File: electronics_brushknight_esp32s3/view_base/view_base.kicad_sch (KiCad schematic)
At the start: 107 parts, among them J1 BLDC, J2 USB_C_Receptacle_USB2.0, J3 LCD, J4 A, J5 B, Q1 MMBT4403, Q2 UMH3N, U1 MT6701-CT, U10 ESP32-S3-WROOM-1-N8R8, U4 CP2102N-A02-GQFN28, U4 HX711, U5 TMC6300, U7 SN74LV1T34DBV, U8 VEML7700, U9 TS1117BCW33_RPG

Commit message: devkit pcb preview
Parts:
- removed D1, D2, D3, D4, D5, D6, D7, D8: SK6812SIDE-A, cleaned footprints:SK6812-SIDE-A, symbol SK6812:SK6812SIDE-A
- removed H4: MountHole, Holes:MountingHole_2.2mm_M2_ISO7380_Pad_NonVirtual, symbol Mechanical:MountingHole_Pad
- removed Q2: UMH3N, cleaned footprints:SOT-363_SC-70-6, symbol Transistor_BJT:UMH3N
- removed R3: 1K, cleaned footprints:R_0603_1608Metric, symbol Device:R_Small
- removed U4: CP2102N-A02-GQFN28, cp2102:Silicon_Labs-CP2102N-A02-GQFN28-IPC_A, symbol terrarium-rescue:CP2102N-A02-GQFN28-CP2102N-A02-GQFN28
- added C100, C101, C30, C31, C32, C33, C34, C35, C36, C37, C38, C39, C40, C41, C42, C43, C44, C45, C46, C47, C48, C49, C50, C51, C52, C53, C54, C55, C56, C57, C58, C59, C60, C61, C62, C63, C64, C65, C66, C67, C68, C69, C70, C71, C72, C73, C74, C75, C76, C77, C79, C80, C81, C82, C88, C90, C92, C94, C95, C96, C97, C98, C99: 0.1uF, cleaned footprints:C_0402_1005Metric, symbol Device:C_Small
- added C27, C38: 10uF, smd_clean:C_0603_1608Metric, symbol Device:C_Small
- added C39: 100nF, smd_clean:C_0603_1608Metric, symbol Device:C_Small
- added D10, D11, D12, D13, D14, D15, D16, D17, D18, D19, D20, D21, D22, D23, D24, D25, D26, D27, D28, D29, D30, D31, D32, D33, D34, D35, D36, D37, D38, D39, D40, D41, D42, D43, D44, D45, D46, D47, D48, D49, D50, D51, D52, D53, D54, D55, D56, D57, D58, D59, D60, D61, D62, D63, D64, D65, D66, D67, D68, D69, D70, D71, D72, D73, D74, D75, D76, D77, D78, D79, D80, D9: SK6805, cleaned footprints:LED_SK6812_EC15_1.5x1.5mm, symbol LED:SK6812
- added J6: LCD - FPC, screen_connector:Amphenol FCI FPC 8 pin 0.5 pitch, symbol Connector_Generic:Conn_01x08
- added J7, J8, J9: Conn_01x04_Socket, cleaned footprints:JST_SH_SM04B-SRSS-TB_1x04-1MP_P1.00mm_Horizontal, symbol Connector:Conn_01x04_Socket
- added Q4, Q5: BSS138, smd_clean:SOT-23, symbol Transistor_FET:BSS138
- added R18, R19, R20, R21, R22, R23: 10K, smd_clean:R_0603_1608Metric, symbol Device:R_Small
- added R28: 10k, cleaned footprints:R_0603_1608Metric, symbol Device:R_Small
- added SW1: RST, smd_clean:SW_SPST_PTS810, symbol Switch:SW_Push
- added SW2: Boot, smd_clean:SW_SPST_PTS810, symbol Switch:SW_Push
- added TP17: IO40, cleaned footprints:TestPoint_Pad_D2.0mm_ValueSilk, symbol Connector:TestPoint_Small
- added TP18: IO41, cleaned footprints:TestPoint_Pad_D2.0mm_ValueSilk, symbol Connector:TestPoint_Small
- added TP19: IO42, cleaned footprints:TestPoint_Pad_D2.0mm_ValueSilk, symbol Connector:TestPoint_Small
- added TP20: IO45, cleaned footprints:TestPoint_Pad_D2.0mm_ValueSilk, symbol Connector:TestPoint_Small
- added TP21: IO46, cleaned footprints:TestPoint_Pad_D2.0mm_ValueSilk, symbol Connector:TestPoint_Small
- added TP22: IO47, cleaned footprints:TestPoint_Pad_D2.0mm_ValueSilk, symbol Connector:TestPoint_Small
- added TP23: IO48, cleaned footprints:TestPoint_Pad_D2.0mm_ValueSilk, symbol Connector:TestPoint_Small
- added U2: USBLC6-2SC6, smd_clean:SOT-23-6, symbol Power_Protection:USBLC6-2SC6
- added U7: VL53L0CXV0DH_1, smd_clean:LGA12_1, symbol VL53L0CXV0DH_1:VL53L0CXV0DH_1
- added U8: LP5907MFX-2.8, cleaned footprints:SOT-23-5, symbol Regulator_Linear:LP5907MFX-2.8
- C1, C11, C2, C29, C3, C4, C5, C6, C7, C8: footprint cleaned footprints:C_0603_1608Metric -> cleaned footprints:C_0402_1005Metric; Digikey 1276-1935-1-ND -> (none); LCSC C1591 -> C83056; Mouser 187-CL10B104KB8NNWC -> (none)
- TP1, TP10, TP11, TP12, TP13, TP14, TP15, TP16, TP3, TP4, TP5, TP6, TP7, TP8, TP9: footprint Modified:TestPoint_Pad_D2.0mm_ValueSilk -> cleaned footprints:TestPoint_Pad_D2.0mm_ValueSilk
- TP2: value 3.3v -> 3V3; footprint Modified:TestPoint_Pad_D2.0mm_ValueSilk -> cleaned footprints:TestPoint_Pad_D2.0mm_ValueSilk
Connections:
- net +3V3: now also C27.2, J6.1 (Pin_1), R20.2, R21.2, R28.1, U8.1 (IN), U8.3 (EN); no longer C11.1
- net +5V: now also C11.1, C100.1, C101.1, C30.1, C31.1, C32.1, C33.1, C34.1, C35.1, C36.1, C37.1, C38.1, C39.1, C40.1, C41.1, C42.1, C43.1, C44.1, C45.1, C46.1, C47.1, C48.1, C49.1, C50.1, C51.1, C52.1, C53.1, C54.1, C55.1, C56.1, C57.1, C58.1, C59.1, C60.1, C61.1, C62.1, C63.1, C64.1, C65.1, C66.1, C67.1, C68.1, C69.1, C70.1, C71.1, C72.1, C73.1, C74.1, C75.1, C76.1, C77.1, C79.1, C80.1, C81.1, C82.1, C88.1, C90.1, C92.1, C94.1, C95.1, C96.1, C97.1, C98.1, C99.1, D10.3 (VDD), D11.3 (VDD), D12.3 (VDD), D13.3 (VDD), D14.3 (VDD), D15.3 (VDD), D16.3 (VDD), D17.3 (VDD), D18.3 (VDD), D19.3 (VDD), D20.3 (VDD), D21.3 (VDD), D22.3 (VDD), D23.3 (VDD), D24.3 (VDD), D25.3 (VDD), D26.3 (VDD), D27.3 (VDD), D28.3 (VDD), D29.3 (VDD), D30.3 (VDD), D31.3 (VDD), D32.3 (VDD), D33.3 (VDD), D34.3 (VDD), D35.3 (VDD), D36.3 (VDD), D37.3 (VDD), D38.3 (VDD), D39.3 (VDD), D40.3 (VDD), D41.3 (VDD), D42.3 (VDD), D43.3 (VDD), D44.3 (VDD), D45.3 (VDD), D46.3 (VDD), D47.3 (VDD), D48.3 (VDD), D49.3 (VDD), D50.3 (VDD), D51.3 (VDD), D52.3 (VDD), D53.3 (VDD), D54.3 (VDD), D55.3 (VDD), D56.3 (VDD), D57.3 (VDD), D58.3 (VDD), D59.3 (VDD), D60.3 (VDD), D61.3 (VDD), D62.3 (VDD), D63.3 (VDD), D64.3 (VDD), D65.3 (VDD), D66.3 (VDD), D67.3 (VDD), D68.3 (VDD), D69.3 (VDD), D70.3 (VDD), D71.3 (VDD), D72.3 (VDD), D73.3 (VDD), D74.3 (VDD), D75.3 (VDD), D76.3 (VDD), D77.3 (VDD), D78.3 (VDD), D79.3 (VDD), D80.3 (VDD), D9.3 (VDD), J7.3 (Pin_3), J8.3 (Pin_3), J9.3 (Pin_3), U2.5 (VBUS)
- net ESP32_BOOT: now also R28.2, SW2.1
- net ESP32_EN: now also SW1.1
- net GND: now also C100.2, C101.2, C27.1, C30.2, C31.2, C32.2, C33.2, C34.2, C35.2, C36.2, C37.2, C38.1, C38.2, C39.1, C39.2, C40.2, C41.2, C42.2, C43.2, C44.2, C45.2, C46.2, C47.2, C48.2, C49.2, C50.2, C51.2, C52.2, C53.2, C54.2, C55.2, C56.2, C57.2, C58.2, C59.2, C60.2, C61.2, C62.2, C63.2, C64.2, C65.2, C66.2, C67.2, C68.2, C69.2, C70.2, C71.2, C72.2, C73.2, C74.2, C75.2, C76.2, C77.2, C79.2, C80.2, C81.2, C82.2, C88.2, C90.2, C92.2, C94.2, C95.2, C96.2, C97.2, C98.2, C99.2, D10.1 (VSS), D11.1 (VSS), D12.1 (VSS), D13.1 (VSS), D14.1 (VSS), D15.1 (VSS), D16.1 (VSS), D17.1 (VSS), D18.1 (VSS), D19.1 (VSS), D20.1 (VSS), D21.1 (VSS), D22.1 (VSS), D23.1 (VSS), D24.1 (VSS), D25.1 (VSS), D26.1 (VSS), D27.1 (VSS), D28.1 (VSS), D29.1 (VSS), D30.1 (VSS), D31.1 (VSS), D32.1 (VSS), D33.1 (VSS), D34.1 (VSS), D35.1 (VSS), D36.1 (VSS), D37.1 (VSS), D38.1 (VSS), D39.1 (VSS), D40.1 (VSS), D41.1 (VSS), D42.1 (VSS), D43.1 (VSS), D44.1 (VSS), D45.1 (VSS), D46.1 (VSS), D47.1 (VSS), D48.1 (VSS), D49.1 (VSS), D50.1 (VSS), D51.1 (VSS), D52.1 (VSS), D53.1 (VSS), D54.1 (VSS), D55.1 (VSS), D56.1 (VSS), D57.1 (VSS), D58.1 (VSS), D59.1 (VSS), D60.1 (VSS), D61.1 (VSS), D62.1 (VSS), D63.1 (VSS), D64.1 (VSS), D65.1 (VSS), D66.1 (VSS), D67.1 (VSS), D68.1 (VSS), D69.1 (VSS), D70.1 (VSS), D71.1 (VSS), D72.1 (VSS), D73.1 (VSS), D74.1 (VSS), D75.1 (VSS), D76.1 (VSS), D77.1 (VSS), D78.1 (VSS), D79.1 (VSS), D80.1 (VSS), D9.1 (VSS), J6.2 (Pin_2), J7.4 (Pin_4), J8.4 (Pin_4), J9.4 (Pin_4), SW1.2, SW2.2, U2.2 (GND), U7.12 (GND4), U7.2 (AVSSVCSEL), U7.3 (GND), U7.4 (GND2), U7.6 (GND3), U8.2 (GND)
- net LCD_BACKLIGHT: now also J6.6 (Pin_6)
- net LCD_CMD: now also J6.8 (Pin_8)
- net LCD_CS: now also J6.7 (Pin_7)
- net LCD_DATA: now also J6.5 (Pin_5)
- net LCD_RST: now also U10.18 (IO10), J6.3 (Pin_3); no longer U10.6 (IO6)
- net LCD_SCK: now also J6.4 (Pin_4)
- net LED_DATA_3V3: now also U10.20 (IO12); no longer U10.7 (IO7)
- net LED_DATA_5V: now also D9.2 (DIN)
- net MAG_CSN: now also U10.19 (IO11); no longer U10.22 (IO14)
- net MAG_DO: now also U10.22 (IO14); no longer U10.30 (IO37)
- net SCL: now also U10.31 (IO38), J7.1 (Pin_1), J8.1 (Pin_1), J9.1 (Pin_1), Q4.3 (D), R21.1; no longer U10.12 (IO8)
- net SDA: now also U10.32 (IO39), J7.2 (Pin_2), J8.2 (Pin_2), J9.2 (Pin_2), Q5.3 (D), R20.1; no longer U10.8 (IO15)
- net STRAIN_DO: now also U10.23 (IO21); no longer U10.31 (IO38)
- net TMC_DIAG: now also U10.6 (IO6); no longer U10.29 (IO36)
- net TMC_UH: now also U10.12 (IO8); no longer U10.14 (IO20)
- net TMC_UL: now also U10.9 (IO16); no longer U10.13 (IO19)
- net TMC_VH: now also U10.11 (IO18); no longer U10.23 (IO21)
- net TMC_VL: now also U10.7 (IO7); no longer U10.10 (IO17)
- net TMC_WH: now also U10.10 (IO17); no longer U10.20 (IO12)
- net TMC_WL: now also U10.8 (IO15); no longer U10.11 (IO18)
- net USB_D+: now also U2.3 (I/O2)
- net USB_D-: now also U2.1 (I/O1)
- net at U10.16 (IO46): now also TP21.1
- net at U10.24 (IO47): now also TP22.1
- net at U10.25 (IO48): now also TP23.1
- net at U10.26 (IO45): now also TP20.1
- net at U10.33 (IO40): now also TP17.1
- net at U10.34 (IO41): now also TP18.1
- net at U10.35 (IO42): now also TP19.1
- new net: D27.4 (DOUT), D28.2 (DIN)
- new net: D28.4 (DOUT), D29.2 (DIN)
- new net: D19.4 (DOUT), D20.2 (DIN)
- new net: D20.4 (DOUT), D21.2 (DIN)
- new net: D16.4 (DOUT), D17.2 (DIN)
- new net: D17.4 (DOUT), D18.2 (DIN)
- new net: D34.4 (DOUT), D35.2 (DIN)
- new net: D35.4 (DOUT), D36.2 (DIN)
- new net: D36.4 (DOUT), D37.2 (DIN)
- new net: R19.1, U7.7 (GPIO1)
- new net: D48.4 (DOUT), D52.2 (DIN)
- new net: D52.4 (DOUT), D56.2 (DIN)
- new net: D59.4 (DOUT), D63.2 (DIN)
- new net: D63.4 (DOUT), D67.2 (DIN)
- new net: R18.1, U7.5 (XSHUT)
- new net: D40.4 (DOUT), D41.2 (DIN)
- new net: D41.4 (DOUT), D45.2 (DIN)
- new net: D74.4 (DOUT), D75.2 (DIN)
- new net: D75.4 (DOUT), D76.2 (DIN)
- new net: D24.4 (DOUT), D25.2 (DIN)
- new net: D25.4 (DOUT), D26.2 (DIN)
- new net: D64.4 (DOUT), D68.2 (DIN)
- new net: D68.4 (DOUT), D72.2 (DIN)
- new net: D56.4 (DOUT), D60.2 (DIN)
- new net: D60.4 (DOUT), D64.2 (DIN)
- new net: D49.4 (DOUT), D53.2 (DIN)
- new net: D53.4 (DOUT), D57.2 (DIN)
- new net: D12.4 (DOUT), D13.2 (DIN)
- new net: D13.4 (DOUT), D14.2 (DIN)
- new net: D14.4 (DOUT), D15.2 (DIN)
- new net: D15.4 (DOUT), D16.2 (DIN)
- new net: D61.4 (DOUT), D65.2 (DIN)
- new net: D65.4 (DOUT), D69.2 (DIN)
- new net: D67.4 (DOUT), D71.2 (DIN)
- new net: D44.2 (DIN), D71.4 (DOUT)
- new net: D18.4 (DOUT), D19.2 (DIN)
- new net: D76.4 (DOUT), D77.2 (DIN)
- new net: D77.4 (DOUT), D78.2 (DIN)
- new net: D42.2 (DIN), D69.4 (DOUT)
- new net: D42.4 (DOUT), D46.2 (DIN)
- new net: D46.4 (DOUT), D50.2 (DIN)
- new net: D50.4 (DOUT), D54.2 (DIN)
- new net: D30.4 (DOUT), D31.2 (DIN)
- new net: D31.4 (DOUT), D32.2 (DIN)
- new net: D55.4 (DOUT), D59.2 (DIN)
- new net: D33.4 (DOUT), D34.2 (DIN)
- new net: D26.4 (DOUT), D27.2 (DIN)
- new net: D21.4 (DOUT), D22.2 (DIN)
- new net: D22.4 (DOUT), D23.2 (DIN)
- new net: D44.4 (DOUT), D48.2 (DIN)
- new net: D23.4 (DOUT), D24.2 (DIN)
- new net: D29.4 (DOUT), D30.2 (DIN)
- new net: D78.4 (DOUT), D79.2 (DIN)
- new net: D79.4 (DOUT), D80.2 (DIN)
- new net: D43.4 (DOUT), D47.2 (DIN)
- new net: D47.4 (DOUT), D51.2 (DIN)
- new net: D32.4 (DOUT), D33.2 (DIN)
- new net: D58.4 (DOUT), D62.2 (DIN)
- new net: D62.4 (DOUT), D66.2 (DIN)
- new net: D73.4 (DOUT), D74.2 (DIN)
- new net: D72.4 (DOUT), D73.2 (DIN)
- new net: D43.2 (DIN), D70.4 (DOUT)
- new net: D57.4 (DOUT), D61.2 (DIN)
- new net: D37.4 (DOUT), D38.2 (DIN)
- new net: D39.4 (DOUT), D40.2 (DIN)
- new net: D45.4 (DOUT), D49.2 (DIN)
- new net: D38.4 (DOUT), D39.2 (DIN)
- new net: D66.4 (DOUT), D70.2 (DIN)
- new net: D11.4 (DOUT), D12.2 (DIN)
- new net: D54.4 (DOUT), D58.2 (DIN)
- new net: D10.4 (DOUT), D11.2 (DIN)
- new net: D51.4 (DOUT), D55.2 (DIN)
- new net: D10.2 (DIN), D9.4 (DOUT)
- new net +2V8: C38.2, C39.2, Q4.1 (G), Q5.1 (G), R18.2, R19.2, R22.2, R23.2, U7.1 (AVDDVCSEL), U7.11 (AVDD), U8.5 (OUT)
- new net ESP_USB_D+: U10.14 (IO20), U2.4 (I/O2)
- new net ESP_USB_D-: U10.13 (IO19), U2.6 (I/O1)
- new net SCL_2.8: Q4.2 (S), R23.1, U7.10 (SCL)
- new net SDA_2.8: Q5.2 (S), R22.1, U7.9 (SDA)
- no-connect marks 32 -> 19
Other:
- note added: "Level shifter & pull-ups (Proximity sensor)"
- note added: "Power supply (Proximity sensor)"
- note added: "Proximity sensor"
- note removed: "Reset/Boot via USB serial"
- company: Scott Bezek -> Scott Bezek | Grigorii Merkushev (brushknight)
- moved on the sheet: C26, J3

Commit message: Revert "DevKit PCB"
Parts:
- removed C100, C101, C30, C31, C32, C33, C34, C35, C36, C37, C38, C39, C40, C41, C42, C43, C44, C45, C46, C47, C48, C49, C50, C51, C52, C53, C54, C55, C56, C57, C58, C59, C60, C61, C62, C63, C64, C65, C66, C67, C68, C69, C70, C71, C72, C73, C74, C75, C76, C77, C79, C80, C81, C82, C88, C90, C92, C94, C95, C96, C97, C98, C99: 0.1uF, cleaned footprints:C_0402_1005Metric, symbol Device:C_Small
- removed C27, C38: 10uF, smd_clean:C_0603_1608Metric, symbol Device:C_Small
- removed C39: 100nF, smd_clean:C_0603_1608Metric, symbol Device:C_Small
- removed D10, D11, D12, D13, D14, D15, D16, D17, D18, D19, D20, D21, D22, D23, D24, D25, D26, D27, D28, D29, D30, D31, D32, D33, D34, D35, D36, D37, D38, D39, D40, D41, D42, D43, D44, D45, D46, D47, D48, D49, D50, D51, D52, D53, D54, D55, D56, D57, D58, D59, D60, D61, D62, D63, D64, D65, D66, D67, D68, D69, D70, D71, D72, D73, D74, D75, D76, D77, D78, D79, D80, D9: SK6805, cleaned footprints:LED_SK6812_EC15_1.5x1.5mm, symbol LED:SK6812
- removed J6: LCD - FPC, screen_connector:Amphenol FCI FPC 8 pin 0.5 pitch, symbol Connector_Generic:Conn_01x08
- removed J7, J8, J9: Conn_01x04_Socket, cleaned footprints:JST_SH_SM04B-SRSS-TB_1x04-1MP_P1.00mm_Horizontal, symbol Connector:Conn_01x04_Socket
- removed Q4, Q5: BSS138, smd_clean:SOT-23, symbol Transistor_FET:BSS138
- removed R18, R19, R20, R21, R22, R23: 10K, smd_clean:R_0603_1608Metric, symbol Device:R_Small
- removed R28: 10k, cleaned footprints:R_0603_1608Metric, symbol Device:R_Small
- removed SW1: RST, smd_clean:SW_SPST_PTS810, symbol Switch:SW_Push
- removed SW2: Boot, smd_clean:SW_SPST_PTS810, symbol Switch:SW_Push
- removed TP17: IO40, cleaned footprints:TestPoint_Pad_D2.0mm_ValueSilk, symbol Connector:TestPoint_Small
- removed TP18: IO41, cleaned footprints:TestPoint_Pad_D2.0mm_ValueSilk, symbol Connector:TestPoint_Small
- removed TP19: IO42, cleaned footprints:TestPoint_Pad_D2.0mm_ValueSilk, symbol Connector:TestPoint_Small
- removed TP20: IO45, cleaned footprints:TestPoint_Pad_D2.0mm_ValueSilk, symbol Connector:TestPoint_Small
- removed TP21: IO46, cleaned footprints:TestPoint_Pad_D2.0mm_ValueSilk, symbol Connector:TestPoint_Small
- removed TP22: IO47, cleaned footprints:TestPoint_Pad_D2.0mm_ValueSilk, symbol Connector:TestPoint_Small
- removed TP23: IO48, cleaned footprints:TestPoint_Pad_D2.0mm_ValueSilk, symbol Connector:TestPoint_Small
- removed U2: USBLC6-2SC6, smd_clean:SOT-23-6, symbol Power_Protection:USBLC6-2SC6
- removed U7: VL53L0CXV0DH_1, smd_clean:LGA12_1, symbol VL53L0CXV0DH_1:VL53L0CXV0DH_1
- removed U8: LP5907MFX-2.8, cleaned footprints:SOT-23-5, symbol Regulator_Linear:LP5907MFX-2.8
- added D1, D2, D3, D4, D5, D6, D7, D8: SK6812SIDE-A, cleaned footprints:SK6812-SIDE-A, symbol SK6812:SK6812SIDE-A
- added H4: MountHole, Holes:MountingHole_2.2mm_M2_ISO7380_Pad_NonVirtual, symbol Mechanical:MountingHole_Pad
- added Q2: UMH3N, cleaned footprints:SOT-363_SC-70-6, symbol Transistor_BJT:UMH3N
- added R3: 1K, cleaned footprints:R_0603_1608Metric, symbol Device:R_Small
- added U4: CP2102N-A02-GQFN28, cp2102:Silicon_Labs-CP2102N-A02-GQFN28-IPC_A, symbol terrarium-rescue:CP2102N-A02-GQFN28-CP2102N-A02-GQFN28
- C1, C11, C2, C29, C3, C4, C5, C6, C7, C8: footprint cleaned footprints:C_0402_1005Metric -> cleaned footprints:C_0603_1608Metric; Digikey (none) -> 1276-1935-1-ND; LCSC C83056 -> C1591; Mouser (none) -> 187-CL10B104KB8NNWC
- TP1, TP10, TP11, TP12, TP13, TP14, TP15, TP16, TP3, TP4, TP5, TP6, TP7, TP8, TP9: footprint cleaned footprints:TestPoint_Pad_D2.0mm_ValueSilk -> Modified:TestPoint_Pad_D2.0mm_ValueSilk
- TP2: value 3V3 -> 3.3v; footprint cleaned footprints:TestPoint_Pad_D2.0mm_ValueSilk -> Modified:TestPoint_Pad_D2.0mm_ValueSilk
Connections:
- net ESP_USB_D+ is gone; now on net TMC_UH: U10.14 (IO20)
- net ESP_USB_D- is gone; now on net TMC_UL: U10.13 (IO19)
- net +3V3: now also C11.1, R3.1, U4.6 (VDD), U4.7 (VREGIN), U4.8 (VBUS)
- net +5V: now also D1.2 (VDD), D2.2 (VDD), D3.2 (VDD), D4.2 (VDD), D5.2 (VDD), D6.2 (VDD), D7.2 (VDD), D8.2 (VDD); no longer C11.1
- net ESP32_BOOT: now also Q2.3 (C2)
- net ESP32_EN: now also Q2.6 (C1)
- net GND: now also D1.4 (VSS), D2.4 (VSS), D3.4 (VSS), D4.4 (VSS), D5.4 (VSS), D6.4 (VSS), D7.4 (VSS), D8.4 (VSS), U4.29 (GND), U4.3 (GND)
- net LCD_RST: now also U10.6 (IO6); no longer U10.18 (IO10)
- net LED_DATA_3V3: now also U10.7 (IO7); no longer U10.20 (IO12)
- net LED_DATA_5V: now also D1.1 (DIN)
- net MAG_CSN: now also U10.22 (IO14); no longer U10.19 (IO11)
- net MAG_DO: now also U10.30 (IO37); no longer U10.22 (IO14)
- net SCL: now also U10.12 (IO8); no longer U10.31 (IO38)
- net SDA: now also U10.8 (IO15); no longer U10.32 (IO39)
- net STRAIN_DO: now also U10.31 (IO38); no longer U10.23 (IO21)
- net TMC_DIAG: now also U10.29 (IO36); no longer U10.6 (IO6)
- net TMC_UH: no longer U10.12 (IO8)
- net TMC_UL: no longer U10.9 (IO16)
- net TMC_VH: now also U10.23 (IO21); no longer U10.11 (IO18)
- net TMC_VL: now also U10.10 (IO17); no longer U10.7 (IO7)
- net TMC_WH: now also U10.20 (IO12); no longer U10.10 (IO17)
- net TMC_WL: now also U10.11 (IO18); no longer U10.8 (IO15)
- net USB_D+: now also U4.4 (D+)
- net USB_D-: now also U4.5 (D-)
- net USB_SERIAL_RXI: now also U4.25 (RXD)
- net USB_SERIAL_TXO: now also U4.26 (TXD)
- new net: D1.3 (DOUT), D2.1 (DIN)
- new net: D2.3 (DOUT), D3.1 (DIN)
- new net: D3.3 (DOUT), D4.1 (DIN)
- new net: D4.3 (DOUT), D5.1 (DIN)
- new net: D5.3 (DOUT), D6.1 (DIN)
- new net: D6.3 (DOUT), D7.1 (DIN)
- new net: D7.3 (DOUT), D8.1 (DIN)
- new net: R3.2, U4.9 (~{RST})
- new net DTR: Q2.2 (B1), Q2.4 (E2), U4.28 (DTR)
- new net RTS: Q2.1 (E1), Q2.5 (B2), U4.24 (RTS)
- no-connect marks 19 -> 32
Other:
- note added: "Reset/Boot via USB serial"
- note removed: "Level shifter & pull-ups (Proximity sensor)"
- note removed: "Power supply (Proximity sensor)"
- note removed: "Proximity sensor"
- company: Scott Bezek | Grigorii Merkushev (brushknight) -> Scott Bezek
- moved on the sheet: C26, J3

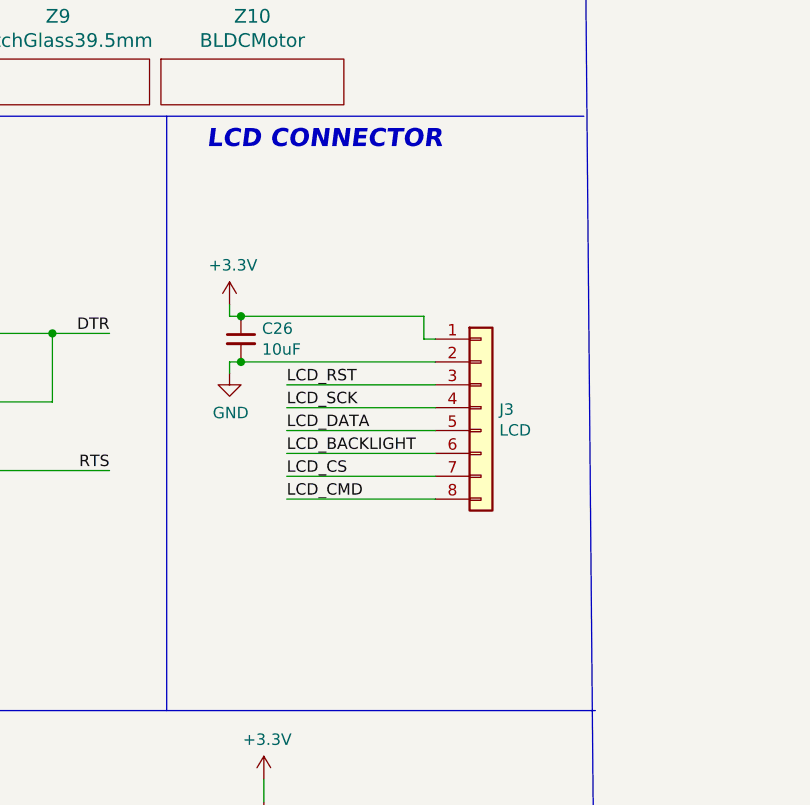
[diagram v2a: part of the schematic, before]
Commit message: wip new display
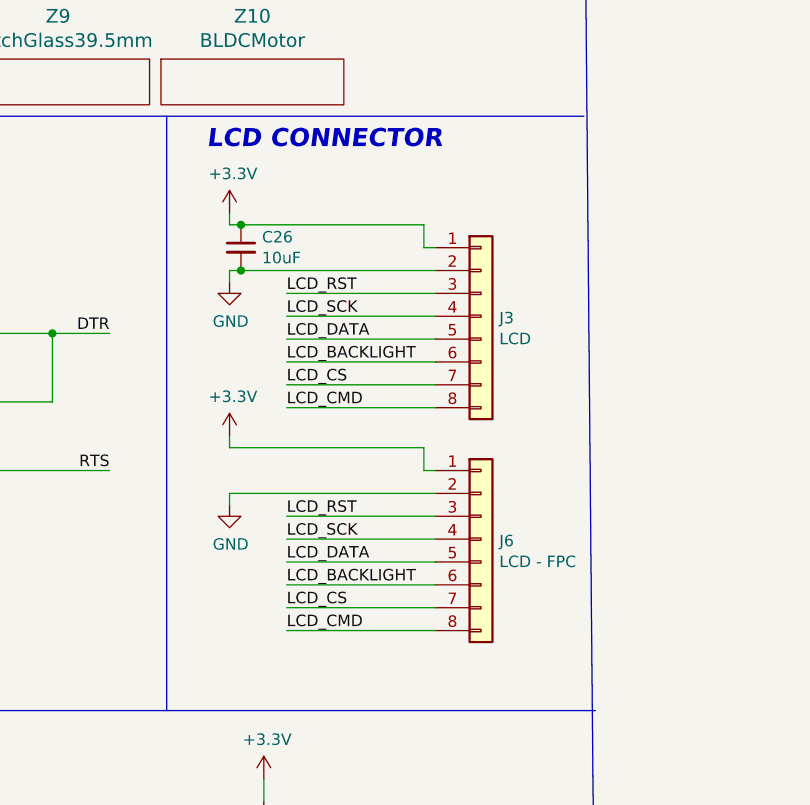
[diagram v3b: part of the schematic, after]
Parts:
- added J6: LCD - FPC, screen_connector:Amphenol FCI FPC 8 pin 0.5 pitch, symbol Connector_Generic:Conn_01x08
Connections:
- net +3V3: now also J6.1 (Pin_1)
- net GND: now also J6.2 (Pin_2)
- net LCD_BACKLIGHT: now also J6.6 (Pin_6)
- net LCD_CMD: now also J6.8 (Pin_8)
- net LCD_CS: now also J6.7 (Pin_7)
- net LCD_DATA: now also J6.5 (Pin_5)
- net LCD_RST: now also J6.3 (Pin_3)
- net LCD_SCK: now also J6.4 (Pin_4)
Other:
- moved on the sheet: C26, J3
